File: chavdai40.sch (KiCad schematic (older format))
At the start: 111 parts, among them J1 Conn_ARM_JTAG_SWD_10, U1 STM32F042K6U6, U2 XC6206P332MR

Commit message: create info.json
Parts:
- D1, D10, D11, D12, D13, D14, D15, D16, D17, D18, D19, D2, D20, D21, D22, D23, D24, D25, D26, D27, D28, D29, D3, D30, D31, D32, D33, D34, D35, D36, D37, D38, D39, D4, D40, D41, D42, D43, D44, D5, D6, D7, D8, D9: footprint Diode_SMD:D_SOD-323F -> Diode_SMD:D_SOD-123

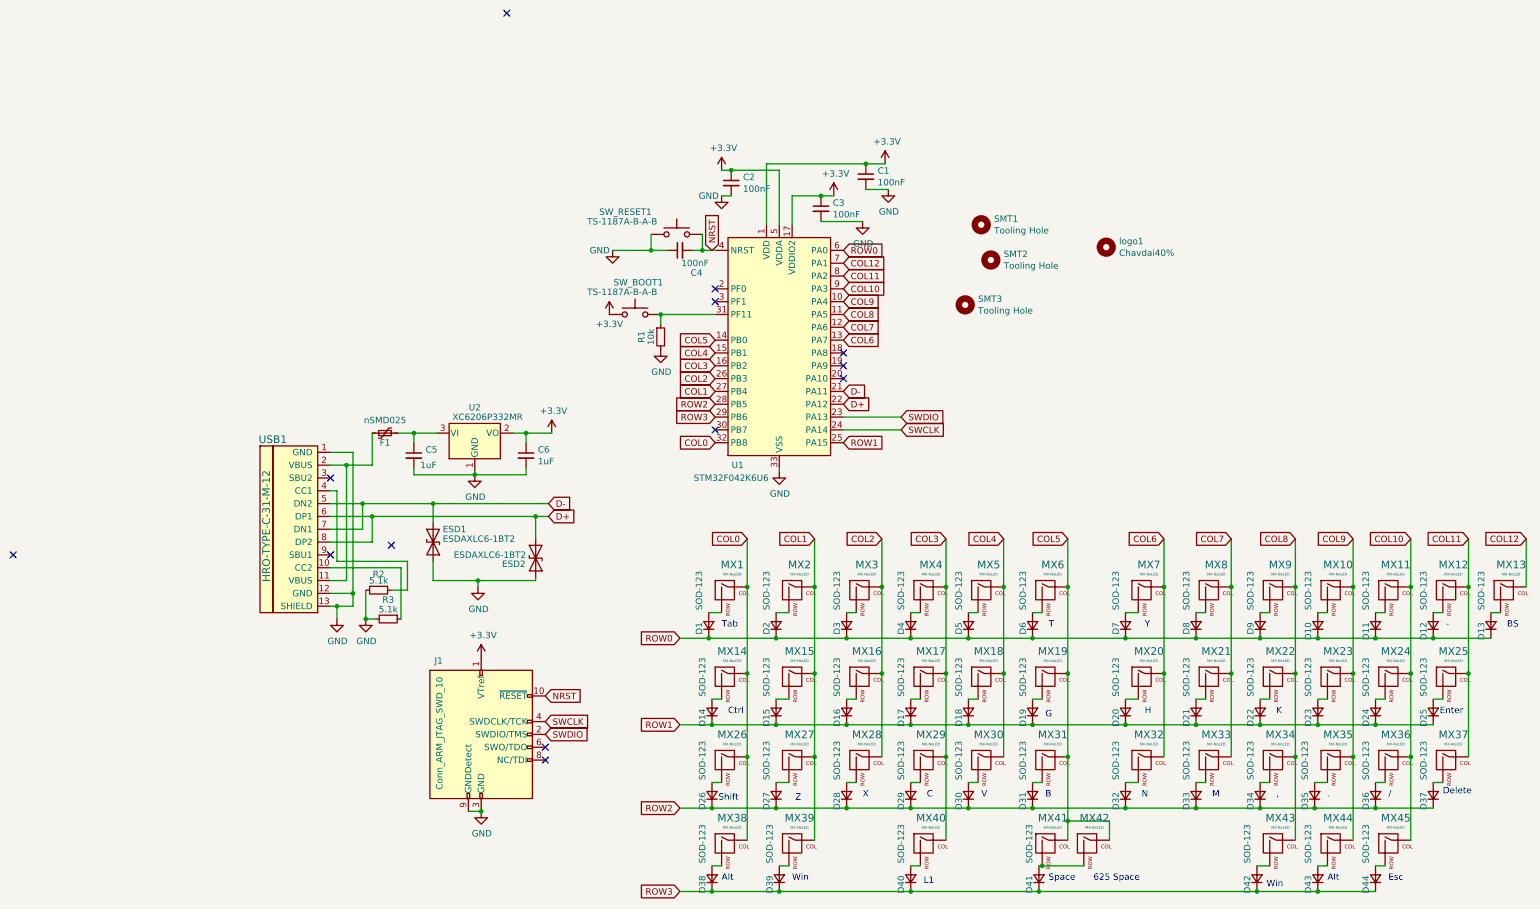
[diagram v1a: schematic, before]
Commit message: update chavdai pcb design(rev2)
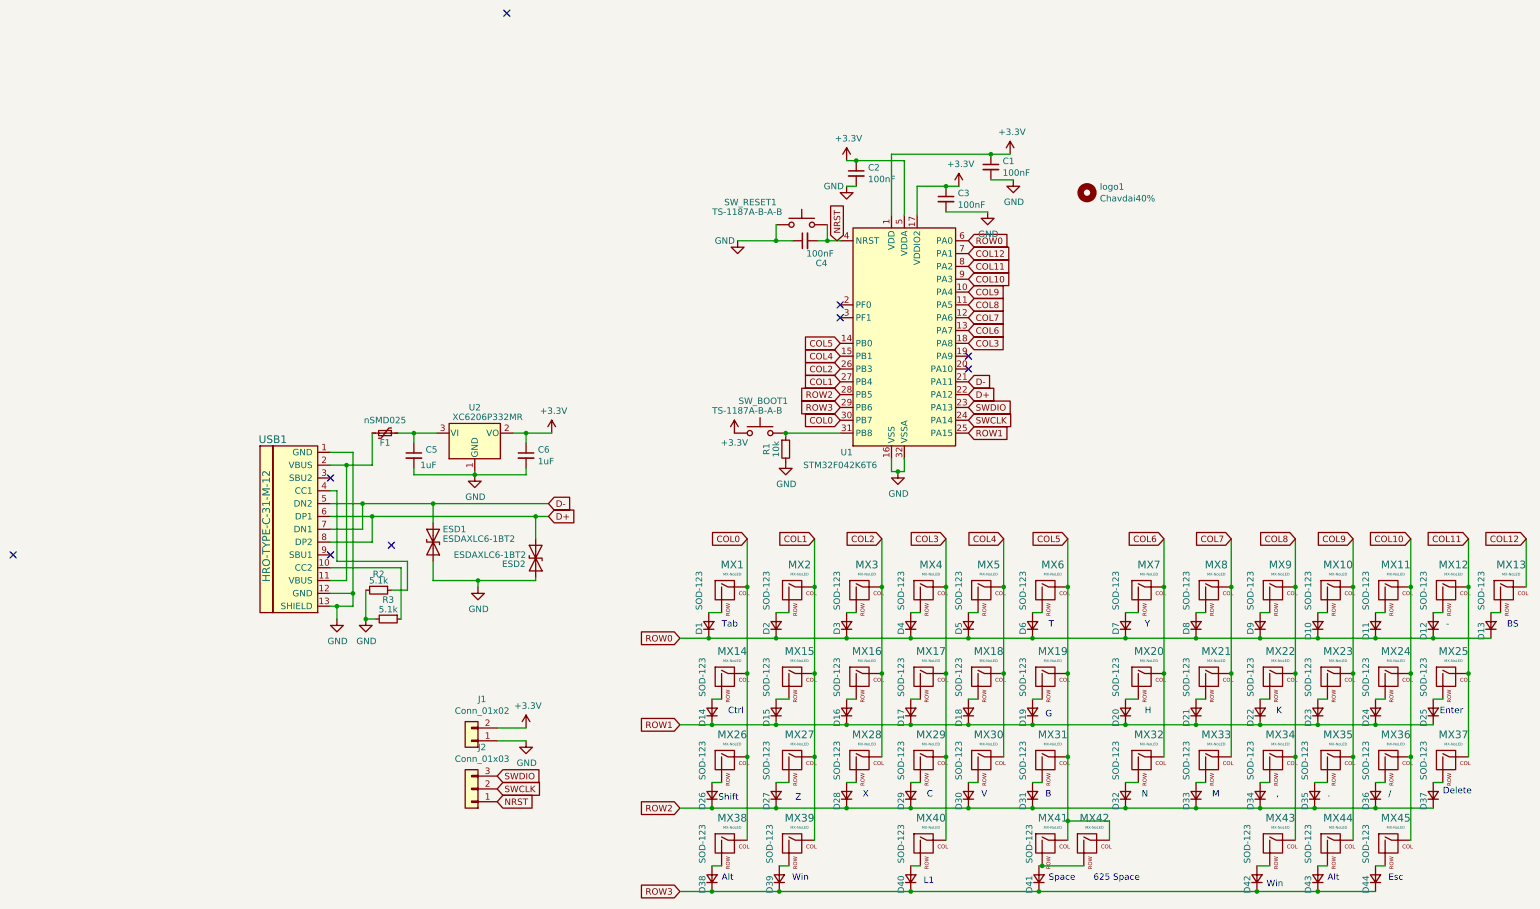
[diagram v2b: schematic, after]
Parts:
- removed J1: Conn_ARM_JTAG_SWD_10, Connector_PinHeader_1.27mm:PinHeader_2x05_P1.27mm_Vertical, symbol Connector:Conn_ARM_JTAG_SWD_10
- removed SMT1, SMT2, SMT3: Tooling Hole, random-keyboard-parts:jlcpcb-tooling-hole, symbol Mechanical:MountingHole
- removed U1: STM32F042K6U6, Package_DFN_QFN:QFN-32-1EP_5x5mm_P0.5mm_EP3.45x3.45mm, symbol MCU_ST_STM32F0:STM32F042K6Ux
- added J1: Conn_01x02, Connector_PinHeader_2.54mm:PinHeader_1x02_P2.54mm_Vertical, symbol Connector_Generic:Conn_01x02
- added J2: Conn_01x03, Connector_PinHeader_2.54mm:PinHeader_1x03_P2.54mm_Vertical, symbol Connector_Generic:Conn_01x03
- added U1: STM32F042K6T6, Package_QFP:LQFP-32_7x7mm_P0.8mm, symbol MCU_ST_STM32F0:STM32F042K6Tx
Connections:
- net +3V3: now also J1.2 (Pin_2), U1.1 (VDD), U1.17 (VDDIO2), U1.5 (VDDA)
- net COL0: now also U1.30 (PB7)
- net COL1: now also U1.27 (PB4)
- net COL10: now also U1.9 (PA3)
- net COL11: now also U1.8 (PA2)
- net COL12: now also U1.7 (PA1)
- net COL2: now also U1.26 (PB3)
- net COL3: now also U1.18 (PA8)
- net COL4: now also U1.15 (PB1)
- net COL5: now also U1.14 (PB0)
- net COL6: now also U1.13 (PA7)
- net COL7: now also U1.12 (PA6)
- net COL8: now also U1.11 (PA5)
- net COL9: now also U1.10 (PA4)
- net D+: now also U1.22 (PA12)
- net D-: now also U1.21 (PA11)
- net GND: now also J1.1 (Pin_1), U1.16 (VSS), U1.32 (VSSA)
- net NRST: now also J2.1 (Pin_1), U1.4 (NRST)
- net ROW0: now also U1.6 (PA0)
- net ROW1: now also U1.25 (PA15)
- net ROW2: now also U1.28 (PB5)
- net ROW3: now also U1.29 (PB6)
- net SWCLK: now also J2.2 (Pin_2), U1.24 (PA14)
- net SWDIO: now also J2.3 (Pin_3), U1.23 (PA13)
- net at R1.1, SW_BOOT1.2: now also U1.31 (PB8)
- no-connect marks 13 -> 9
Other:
- moved on the sheet: C1, C2, C3, C4, R1, SW_BOOT1, SW_RESET1, logo1
